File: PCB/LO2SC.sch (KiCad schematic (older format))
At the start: 0 parts

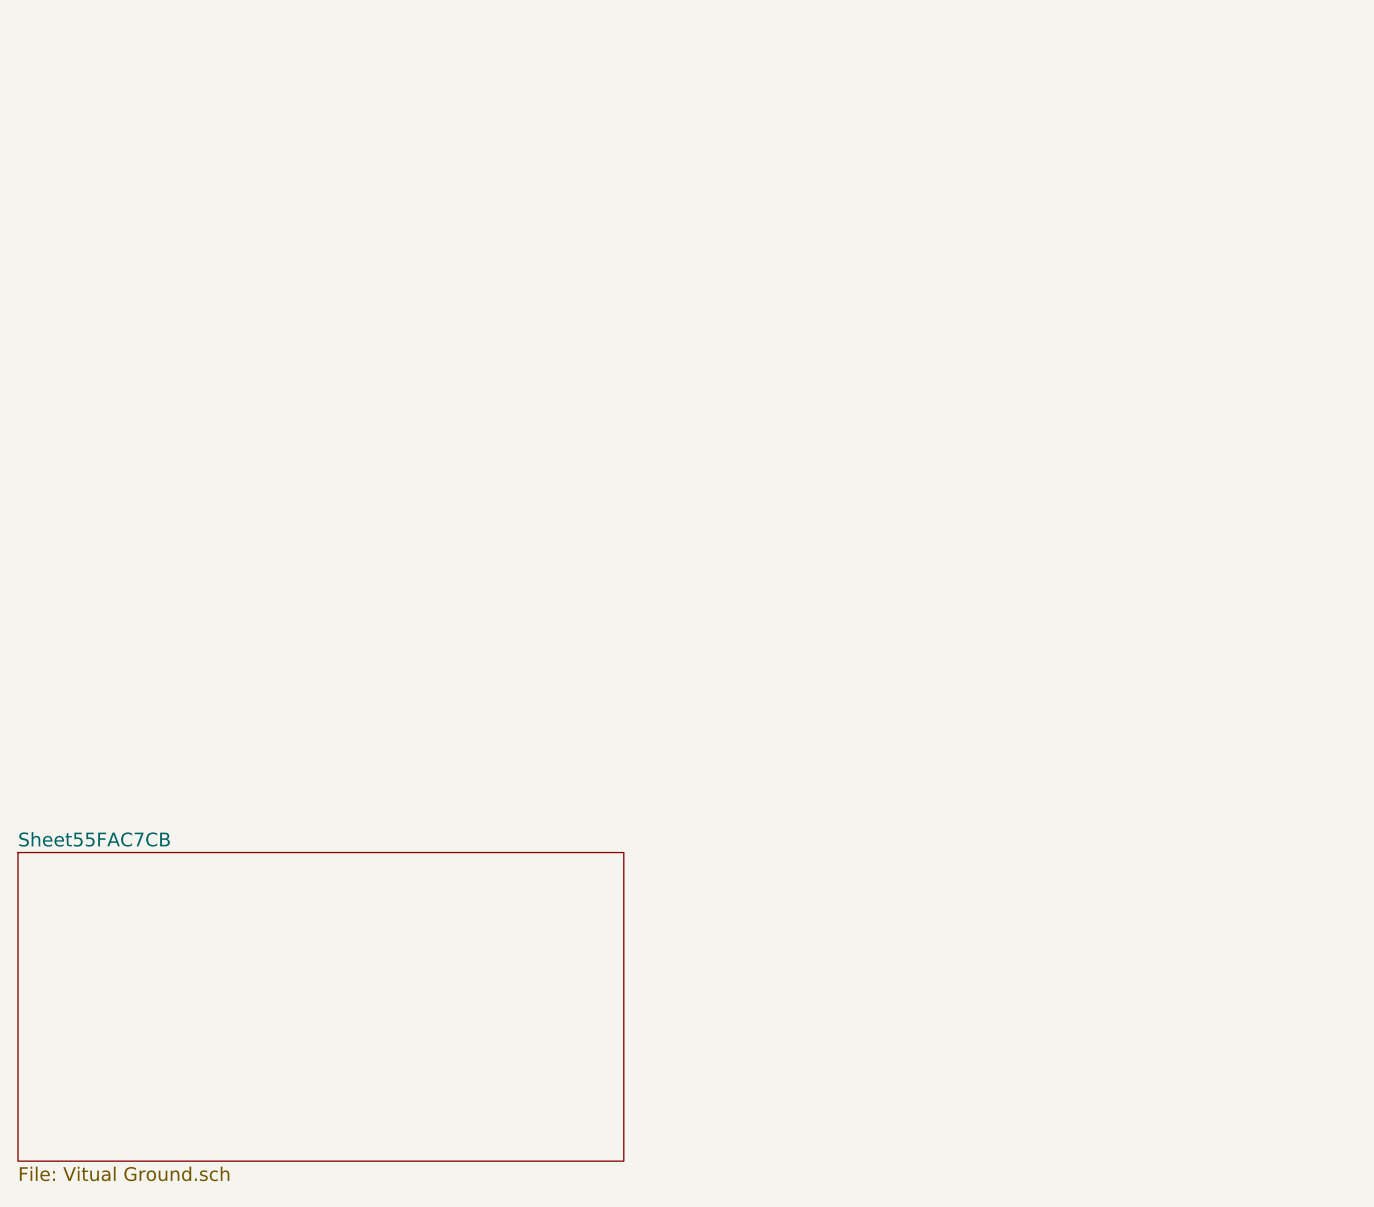
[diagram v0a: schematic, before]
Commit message: - ajout de schematiques
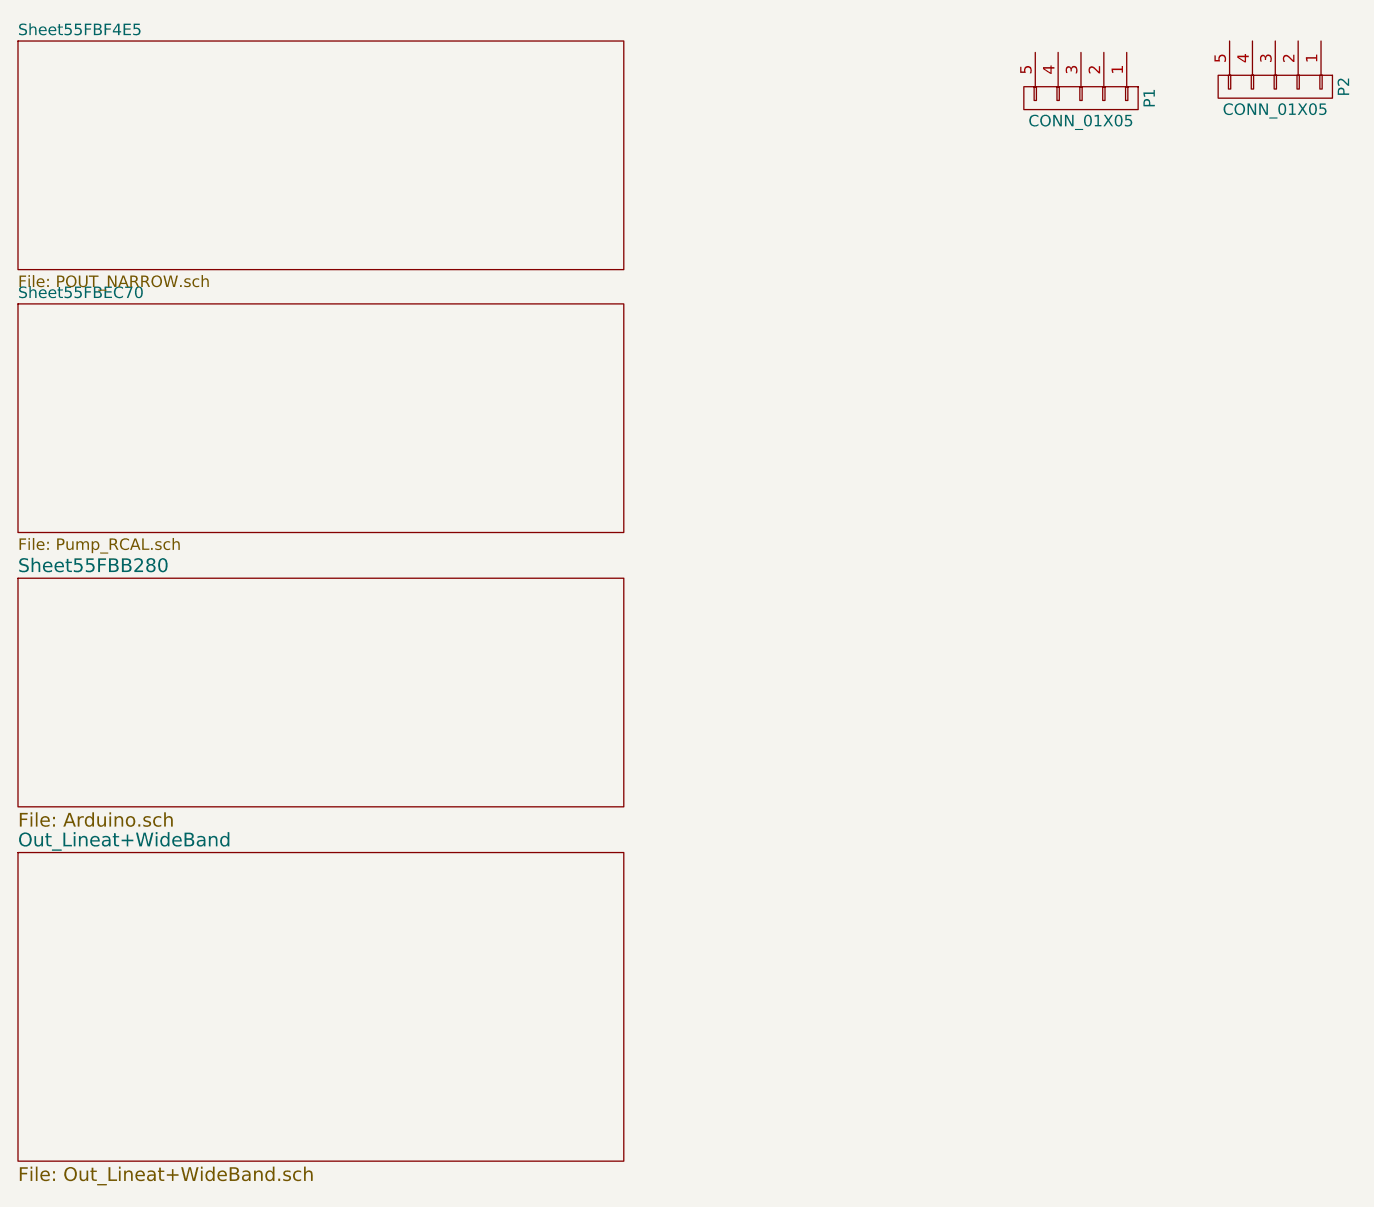
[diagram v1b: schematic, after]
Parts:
- added P1, P2: CONN_01X05, Barrettes:Pin_Header_Straight_1x05, symbol CONN_01X05
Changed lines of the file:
@@
 LIBS:Resistances_SMD_0603
 LIBS:Condensateurs_SMD_0603
+LIBS:Microcontroleur_Atmel_SMD_TQFP
+LIBS:Barrettes_TH
 LIBS:LO2SC-cache
 EELAYER 25 0
@@
 $Descr A4 11693 8268
 encoding utf-8
-Sheet 1 2
+Sheet 1 5
 Title ""
 Date ""
@@
 S 1500 5300 2650 1350
 U 55FAC7CC
-F0 "Sheet55FAC7CB" 60
-F1 "Vitual Ground.sch" 60
+F0 "Out_Lineat+WideBand" 60
+F1 "Out_Lineat+WideBand.sch" 60
 $EndSheet
+$Sheet
+S 1500 4100 2650 1000
+U 55FBB281
+F0 "Sheet55FBB280" 60
+F1 "Arduino.sch" 60
+$EndSheet
+$Sheet
+S 1500 2900 2650 1000
+U 55FBEC71
+F0 "Sheet55FBEC70" 50
+F1 "Pump_RCAL.sch" 50
+$EndSheet
+$Sheet
+S 1500 1750 2650 1000
+U 55FBF4E6
+F0 "Sheet55FBF4E5" 50
+F1 "POUT_NARROW.sch" 50
+$EndSheet
+$Comp
+L CONN_01X05 P1
+U 1 1 55FBF5A3
+P 6150 2000
+F 0 "P1" H 6150 2300 50  0000 C CNN
+F 1 "CONN_01X05" V 6250 2000 50  0000 C CNN
+F 2 "Barrettes:Pin_Header_Straight_1x05" H 6150 2450 60  0001 C CNN
+F 3 "" H 6150 2300 60  0000 C CNN
+F 4 "455-1660-ND" H 6150 2550 50  0001 C CNN "Ref Digikey"
+	1    6150 2000
+	0    1    1    0
+$EndComp
+$Comp
+L CONN_01X05 P2
+U 1 1 55FBF5F9
+P 7000 1950
+F 0 "P2" H 7000 2250 50  0000 C CNN
+F 1 "CONN_01X05" V 7100 1950 50  0000 C CNN
+F 2 "Barrettes:Pin_Header_Straight_1x05" H 7000 2400 60  0001 C CNN
+F 3 "" H 7000 2250 60  0000 C CNN
+F 4 "455-1660-ND" H 7000 2500 50  0001 C CNN "Ref Digikey"
+	1    7000 1950
+	0    1    1    0
+$EndComp
 $EndSCHEMATC
